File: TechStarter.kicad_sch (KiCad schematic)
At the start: 35 parts, among them J1 Conn_01x04_Socket, J10 Conn_01x03_Socket, J11 Conn_01x03_Socket, J12 Conn_01x04_Pin, J2 Conn_01x04_Socket, J3 Conn_01x02_Socket, J4 Conn_01x04_Socket, J5 Conn_01x03_Socket, J6 Conn_01x04_Socket, J7 Conn_01x03_Socket, J8 Conn_01x03_Socket, J9 Conn_01x03_Socket, Q2 IRLZ44N, U1 STM32F446RETx, U2 TMC2209-LA, U3 TMC2209-LA, U5 MX25L3233FM1

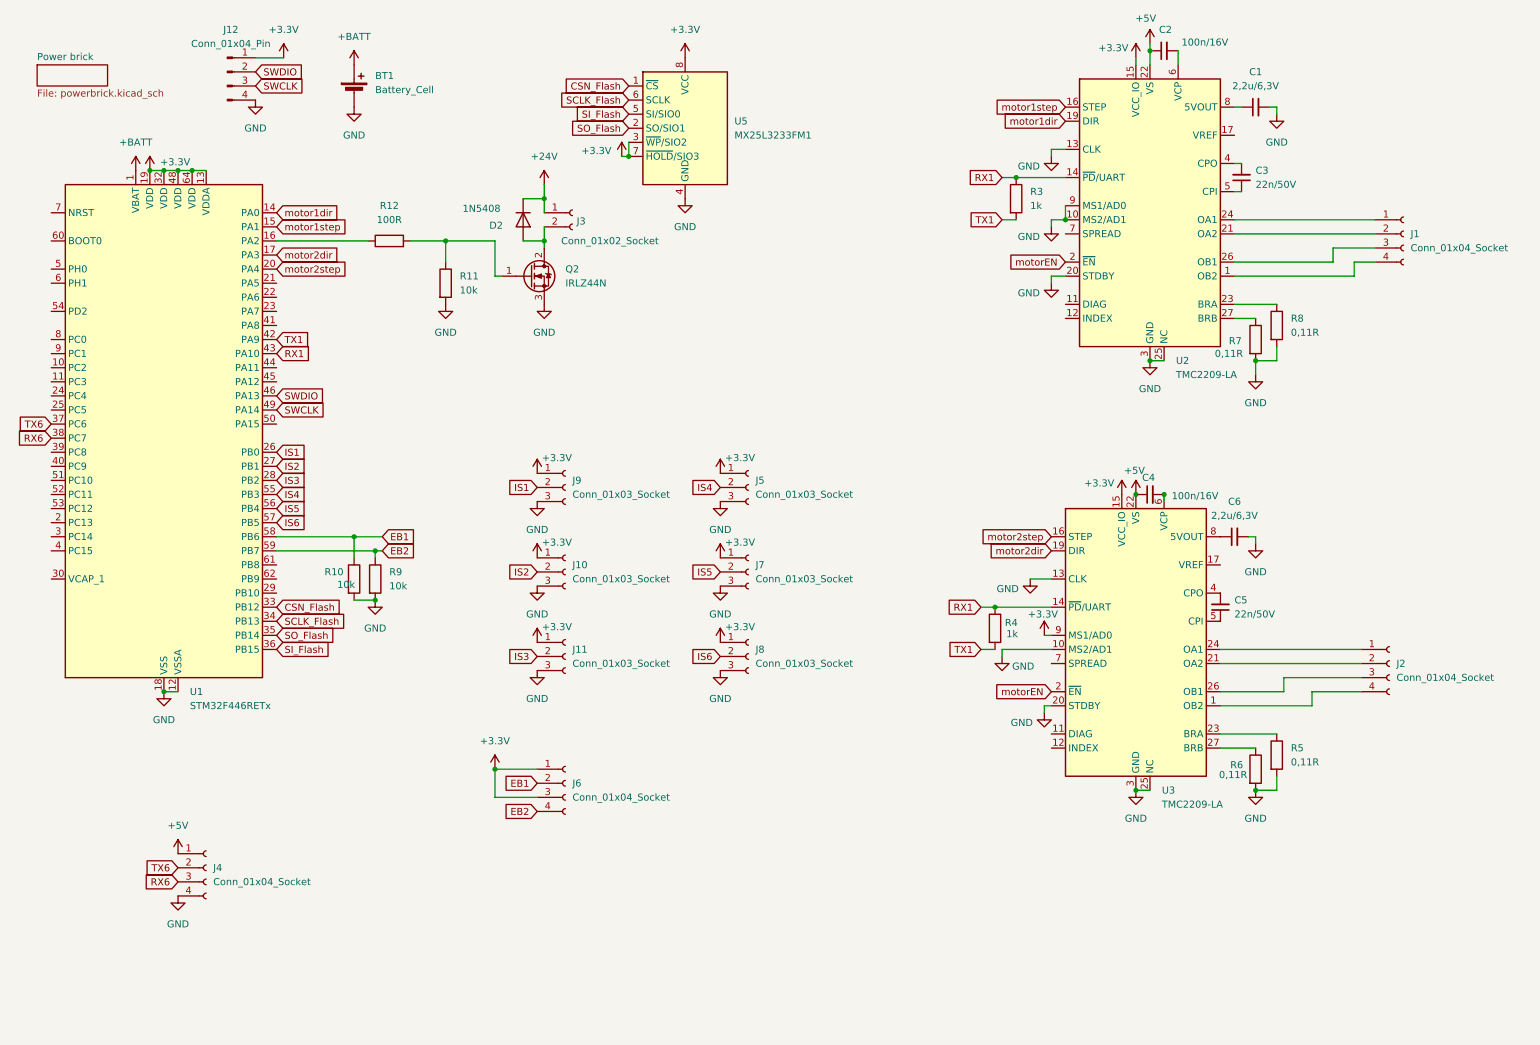
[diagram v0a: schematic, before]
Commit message: .
označení sekcí
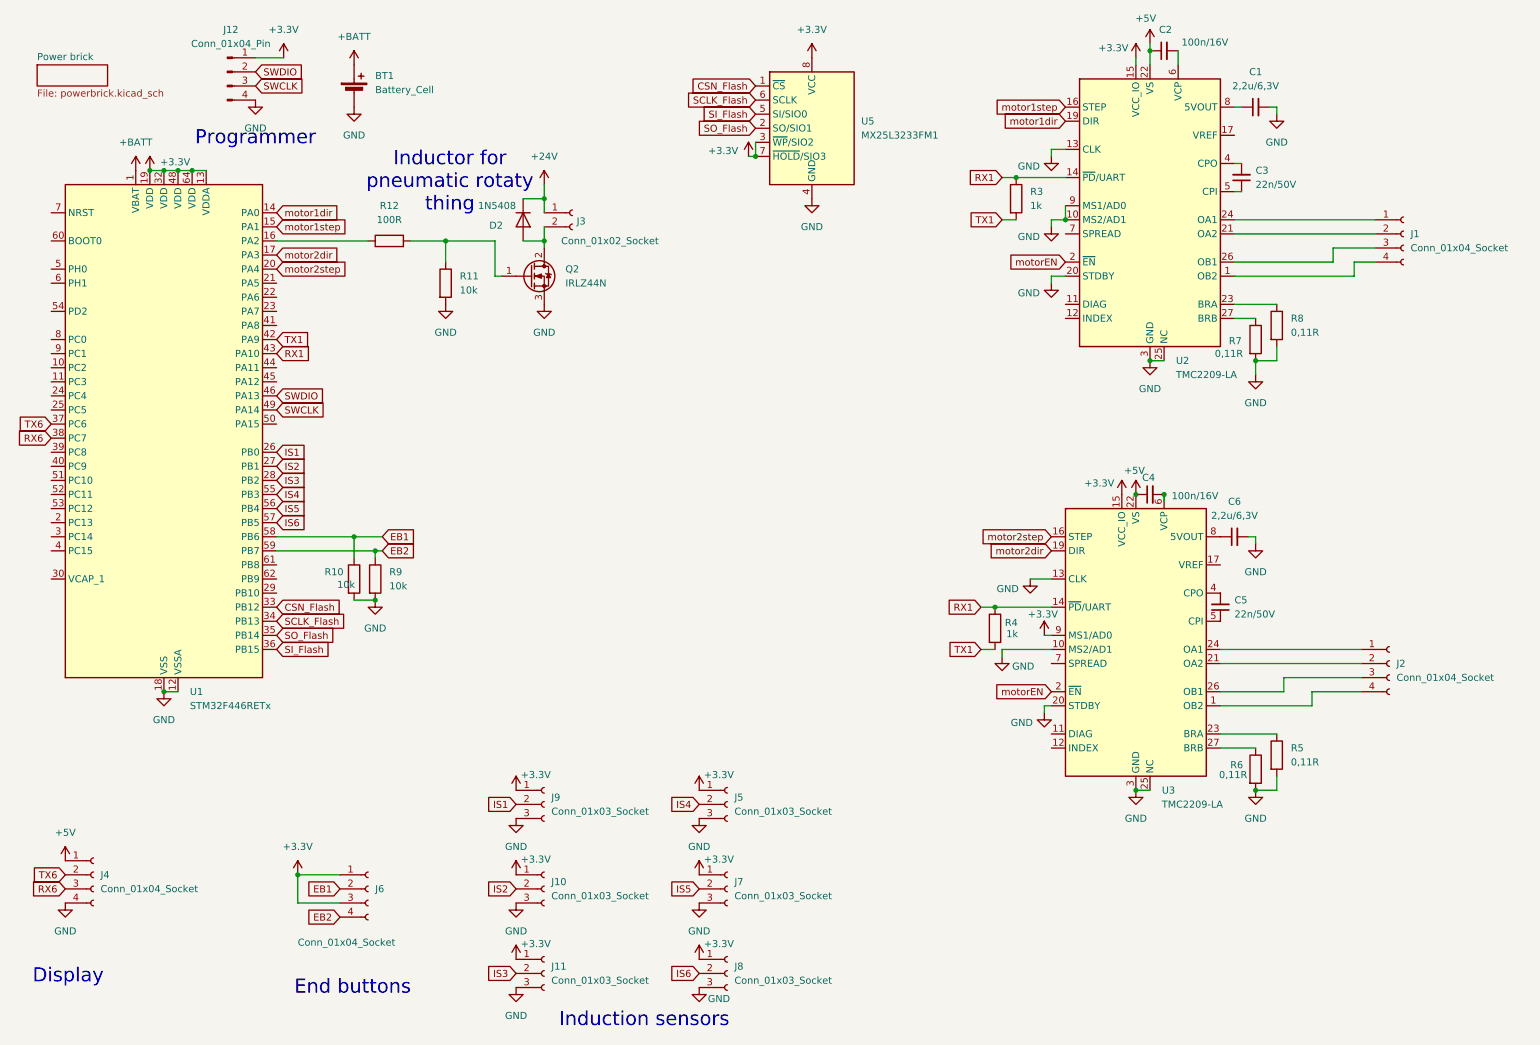
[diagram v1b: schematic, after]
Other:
- note added: "Display"
- note added: "End buttons"
- note added: "Induction sensors"
- note added: "Inductor for pneumatic rotaty thing"
- note added: "Programmer"
- moved on the sheet: J10, J11, J4, J5, J6, J7, J8, J9, U5
